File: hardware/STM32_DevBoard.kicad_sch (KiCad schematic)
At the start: 39 parts, among them SW1 SW_SPST, SW2 SW_MEC_5G, U1 STM32C071CBTx, U2 TP8485E-SR, U3 AZ1117-3.3, U4 HDC1080, U5 SGP40-D-R4

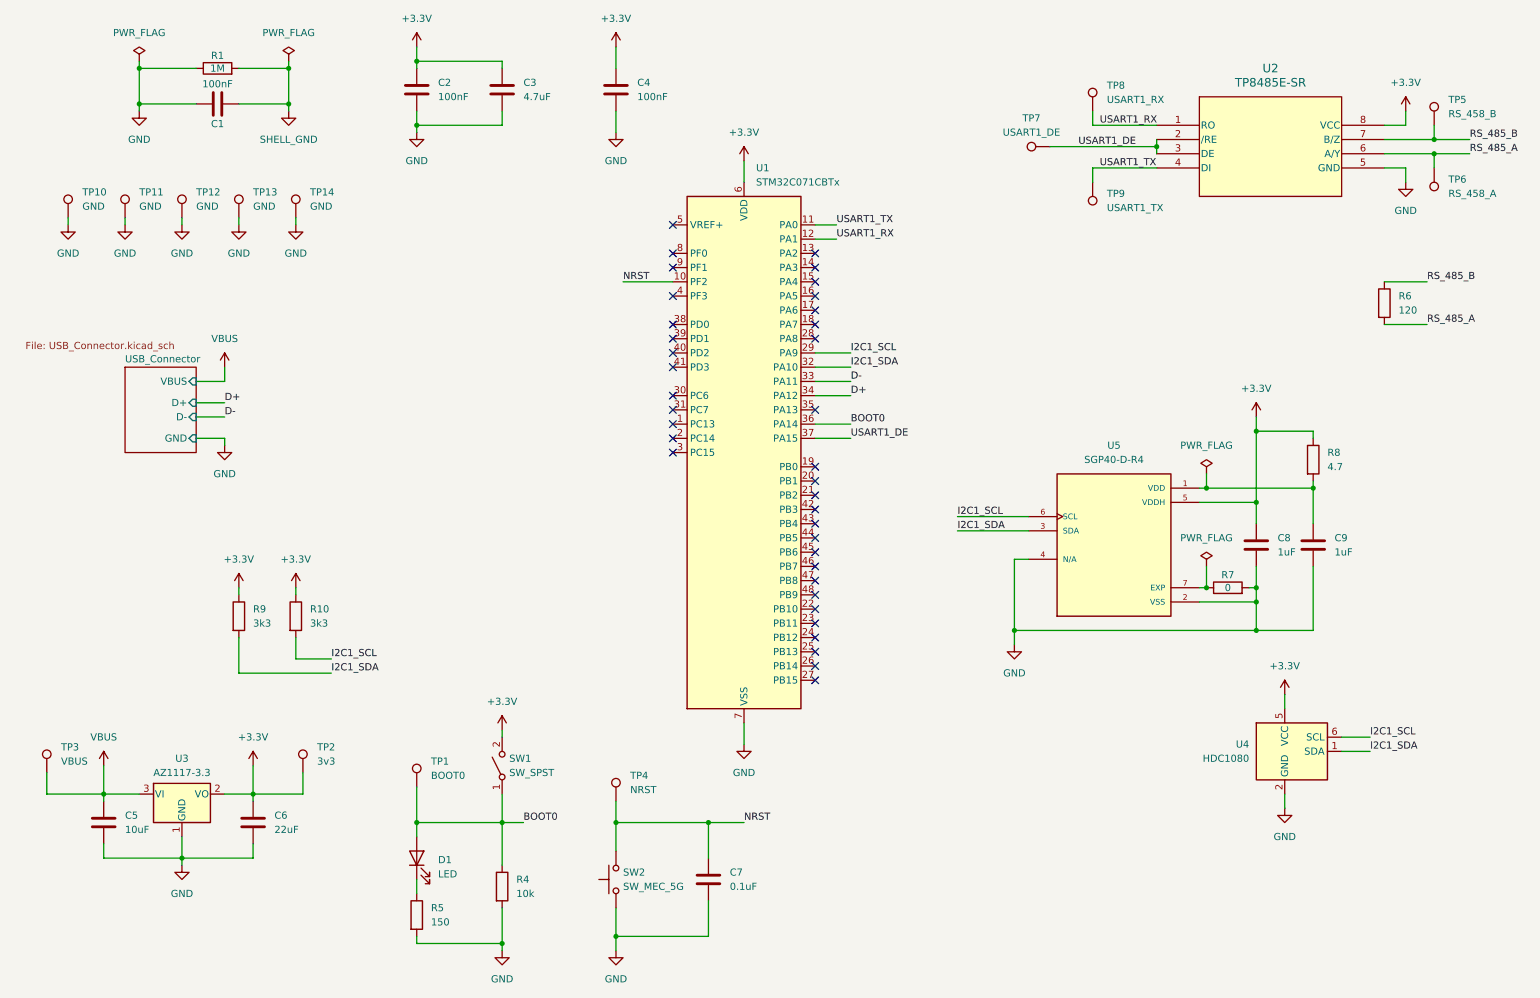
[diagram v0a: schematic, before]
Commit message: encore plein de truc chouette
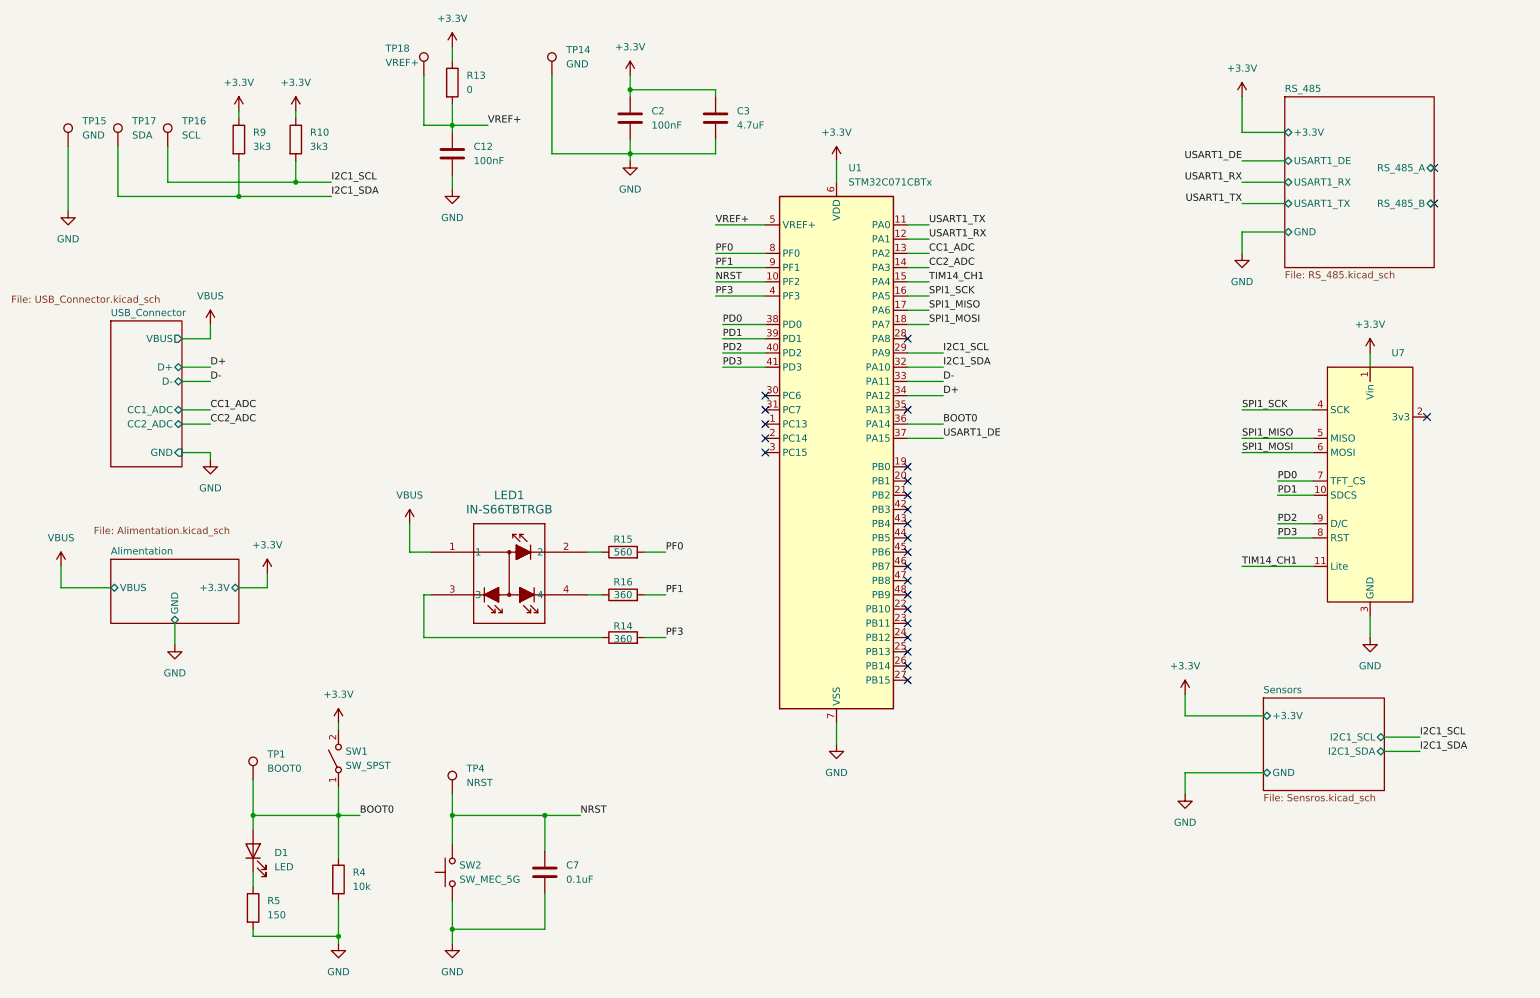
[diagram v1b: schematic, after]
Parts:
- removed C1, C4: 100nF, symbol Device:C
- removed C5: 10uF, symbol Device:C
- removed C6: 22uF, symbol Device:C
- removed C8, C9: 1uF, symbol Device:C
- removed R1: 1M, symbol Device:R
- removed R6: 120, symbol Device:R
- removed R7: 0, symbol Device:R
- removed R8: 4.7, symbol Device:R
- removed TP10, TP11, TP12, TP13: GND, symbol Connector:TestPoint
- removed TP2: 3v3, symbol Connector:TestPoint
- removed TP3: VBUS, symbol Connector:TestPoint
- removed TP5: RS_458_B, symbol Connector:TestPoint
- removed TP6: RS_458_A, symbol Connector:TestPoint
- removed TP7: USART1_DE, symbol Connector:TestPoint
- removed TP8: USART1_RX, symbol Connector:TestPoint
- removed TP9: USART1_TX, symbol Connector:TestPoint
- removed U2: TP8485E-SR, RS_485_FOOT:SO-8SOIC-8_TPK, symbol RS_485_LIB:TP8485E-SR
- removed U3: AZ1117-3.3, Package_TO_SOT_SMD:SOT-223-3_TabPin2, symbol Regulator_Linear:AZ1117-3.3
- removed U4: HDC1080, Package_SON:Texas_PWSON-N6, symbol Sensor_Humidity:HDC1080
- removed U5: SGP40-D-R4, RS_485_FOOT:XCDR_SGP40-D-R4, symbol RS_485_LIB:SGP40-D-R4
- added C12: 100nF, symbol Device:C
- added LED1: IN-S66TBTRGB, RS_485_FOOT:IN-S66TB_INL, symbol RS_485_LIB:IN-S66TBTRGB
- added R13: 0, symbol Device:R
- added R14, R16: 360, symbol Device:R
- added R15: 560, symbol Device:R
- added TP15: GND, symbol Connector:TestPoint
- added TP16: SCL, symbol Connector:TestPoint
- added TP17: SDA, symbol Connector:TestPoint
- added TP18: VREF+, symbol Connector:TestPoint
- added U7: (no value), RS_485_FOOT:TFT_SPI, symbol RS_485_LIB:TFT_SPI
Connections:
- net +3.3V: now also R13.1, U7.1 (Vin)
- net GND: now also C12.2, TP15.1, U7.3 (GND)
- net I2C1_SCL: now also TP16.1
- net I2C1_SDA: now also TP17.1
- net VBUS: now also LED1.1
- net CC1_ADC: now reaches U1.13 (PA2)
- net CC2_ADC: now reaches U1.14 (PA3)
- net TIM14_CH1: now reaches U1.15 (PA4)
- net TIM14_CH1: now also U7.11 (Lite)
- net SPI1_SCK: now reaches U1.16 (PA5)
- net SPI1_SCK: now also U7.4 (SCK)
- net SPI1_MISO: now reaches U1.17 (PA6)
- net SPI1_MISO: now also U7.5 (MISO)
- net SPI1_MOSI: now reaches U1.18 (PA7)
- net SPI1_MOSI: now also U7.6 (MOSI)
- net PD0: now reaches U1.38 (PD0)
- net PD0: now also U7.7 (TFT_CS)
- net PD1: now reaches U1.39 (PD1)
- net PD1: now also U7.10 (SDCS)
- net PF3: now reaches U1.4 (PF3)
- net PF3: now also R14.2
- net PD2: now reaches U1.40 (PD2)
- net PD2: now also U7.9 (D/C)
- net PD3: now reaches U1.41 (PD3)
- net PD3: now also U7.8 (RST)
- net VREF+: now reaches U1.5 (VREF+)
- net VREF+: now also C12.1, R13.2, TP18.1
- net PF0: now reaches U1.8 (PF0)
- net PF0: now also R15.2
- net PF1: now reaches U1.9 (PF1)
- net PF1: now also R16.2
- new net: LED1.3, R14.1
- new net: LED1.2, R15.1
- new net: LED1.4, R16.1
- no-connect marks 37 -> 26
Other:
- added sheet Alimentation (Alimentation.kicad_sch)
- added sheet RS_485 (RS_485.kicad_sch)
- added sheet Sensors (Sensros.kicad_sch)
- sheet USB_Connector ports: added CC1_ADC, CC2_ADC; removed none
- moved on the sheet: C2, C3, C7, D1, R10, R4, R5, R9, SW1, SW2, TP1, TP14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
